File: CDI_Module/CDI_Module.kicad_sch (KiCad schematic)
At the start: 4 parts, among them Q1 TIC226

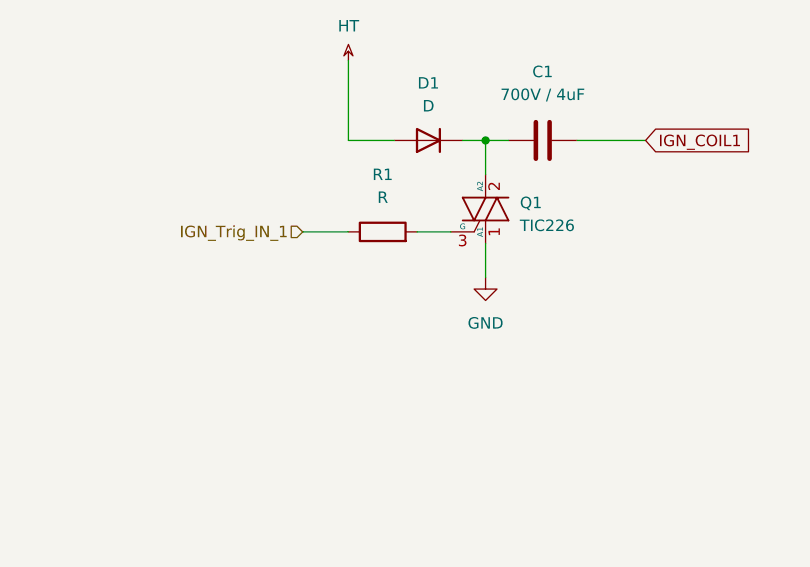
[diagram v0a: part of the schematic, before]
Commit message: First Drawing of High volatage generator part
First Drawing of High volatage generator part
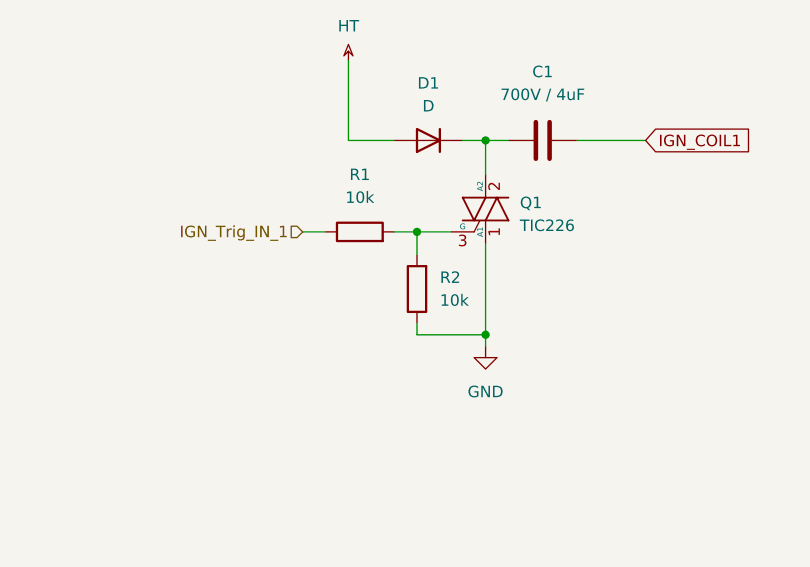
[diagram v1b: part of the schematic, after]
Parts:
- added R2: 10k, Resistor_SMD:R_0603_1608Metric_Pad0.98x0.95mm_HandSolder, symbol Device:R
- R1: value R -> 10k
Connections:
- net GND: now also R2.1
- net at Q1.3 (G), R1.2: now also R2.2
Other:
- moved on the sheet: R1
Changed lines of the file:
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@@
 (kicad_sch (version 20230121) (generator eeschema)
   (paper "A4")
+  (junction (at 91.44 55.88) (diameter 0) (color 0 0 0 0)
+  )
   (junction (at 99.06 45.72) (diameter 0) (color 0 0 0 0)
   )
+  (junction (at 99.06 67.31) (diameter 0) (color 0 0 0 0)
+  )
+  (wire (pts (xy 99.06 67.31) (xy 99.06 68.58))
+    (stroke (width 0) (type default))
+  )
+  (wire (pts (xy 91.44 55.88) (xy 91.44 58.42))
+    (stroke (width 0) (type default))
+  )
   (wire (pts (xy 96.52 45.72) (xy 99.06 45.72))
     (stroke (width 0) (type default))
   )
-  (wire (pts (xy 99.06 57.15) (xy 99.06 60.96))
+  (wire (pts (xy 99.06 57.15) (xy 99.06 67.31))
     (stroke (width 0) (type default))
   )
@@
     (stroke (width 0) (type default))
   )
+  (wire (pts (xy 88.9 55.88) (xy 91.44 55.88))
+    (stroke (width 0) (type default))
+  )
+  (wire (pts (xy 109.22 45.72) (xy 116.84 45.72))
+    (stroke (width 0) (type default))
+  )
   (wire (pts (xy 91.44 55.88) (xy 95.25 55.88))
     (stroke (width 0) (type default))
   )
-  (wire (pts (xy 109.22 45.72) (xy 116.84 45.72))
+  (wire (pts (xy 91.44 67.31) (xy 91.44 66.04))
     (stroke (width 0) (type default))
   )
@@
     (stroke (width 0) (type default))
   )
-  (wire (pts (xy 78.74 55.88) (xy 83.82 55.88))
+  (wire (pts (xy 78.74 55.88) (xy 81.28 55.88))
     (stroke (width 0) (type default))
   )
   (wire (pts (xy 99.06 49.53) (xy 99.06 45.72))
+    (stroke (width 0) (type default))
+  )
+  (wire (pts (xy 91.44 67.31) (xy 99.06 67.31))
     (stroke (width 0) (type default))
   )
@@
     (effects (font (size 1.27 1.27)) (justify right))
   )
-  (symbol (lib_id "Device:R") (at 87.63 55.88 90) (unit 1)
-    (in_bom yes) (on_board yes) (dnp no) (fields_autoplaced)
-    (property "Reference" "R1" (at 87.63 49.53 90)
-      (effects (font (size 1.27 1.27)))
-    )
-    (property "Value" "R" (at 87.63 52.07 90)
-      (effects (font (size 1.27 1.27)))
-    )
-    (property "Footprint" "Resistor_SMD:R_0603_1608Metric_Pad0.98x0.95mm_HandSolder" (at 87.63 57.658 90)
-      (effects (font (size 1.27 1.27)) hide)
-    )
-    (property "Datasheet" "~" (at 87.63 55.88 0)
+  (symbol (lib_id "Device:R") (at 85.09 55.88 90) (unit 1)
+    (in_bom yes) (on_board yes) (dnp no) (fields_autoplaced)
+    (property "Reference" "R1" (at 85.09 49.53 90)
+      (effects (font (size 1.27 1.27)))
+    )
+    (property "Value" "10k" (at 85.09 52.07 90)
+      (effects (font (size 1.27 1.27)))
+    )
+    (property "Footprint" "Resistor_SMD:R_0603_1608Metric_Pad0.98x0.95mm_HandSolder" (at 85.09 57.658 90)
+      (effects (font (size 1.27 1.27)) hide)
+    )
+    (property "Datasheet" "~" (at 85.09 55.88 0)
       (effects (font (size 1.27 1.27)) hide)
     )
@@
     )
   )
-  (symbol (lib_id "power:GND") (at 99.06 60.96 0) (unit 1)
-    (in_bom yes) (on_board yes) (dnp no) (fields_autoplaced)
-    (property "Reference" "#PWR02" (at 99.06 67.31 0)
-      (effects (font (size 1.27 1.27)) hide)
-    )
-    (property "Value" "GND" (at 99.06 66.04 0)
-      (effects (font (size 1.27 1.27)))
-    )
-    (property "Footprint" "" (at 99.06 60.96 0)
-      (effects (font (size 1.27 1.27)) hide)
-    )
-    (property "Datasheet" "" (at 99.06 60.96 0)
+  (symbol (lib_id "power:GND") (at 99.06 68.58 0) (unit 1)
+    (in_bom yes) (on_board yes) (dnp no) (fields_autoplaced)
+    (property "Reference" "#PWR02" (at 99.06 74.93 0)
+      (effects (font (size 1.27 1.27)) hide)
+    )
+    (property "Value" "GND" (at 99.06 73.66 0)
+      (effects (font (size 1.27 1.27)))
+    )
+    (property "Footprint" "" (at 99.06 68.58 0)
+      (effects (font (size 1.27 1.27)) hide)
+    )
+    (property "Datasheet" "" (at 99.06 68.58 0)
       (effects (font (size 1.27 1.27)) hide)
     )
@@
         )
       )
+    )
+  )
+  (symbol (lib_id "Device:R") (at 91.44 62.23 180) (unit 1)
+    (in_bom yes) (on_board yes) (dnp no) (fields_autoplaced)
+    (property "Reference" "R2" (at 93.98 60.96 0)
+      (effects (font (size 1.27 1.27)) (justify right))
+    )
+    (property "Value" "10k" (at 93.98 63.5 0)
+      (effects (font (size 1.27 1.27)) (justify right))
+    )
+    (property "Footprint" "Resistor_SMD:R_0603_1608Metric_Pad0.98x0.95mm_HandSolder" (at 93.218 62.23 90)
+      (effects (font (size 1.27 1.27)) hide)
+    )
+    (property "Datasheet" "~" (at 91.44 62.23 0)
+      (effects (font (size 1.27 1.27)) hide)
+    )
+    (pin "1")
+    (pin "2")
+    (instances
+      (project "CDI_Module"
+        (path "/a4713233-3633-4d06-9186-8236551fb01a"
+          (reference "R2") (unit 1)
+        )
+      )
